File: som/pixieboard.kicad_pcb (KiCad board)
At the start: 8 copper layers, 50 x 50 mm, 11 parts, among them U1 XC7A200T-3FBG484E, U2 AS4C256M16D3, U3 AS4C256M16D3

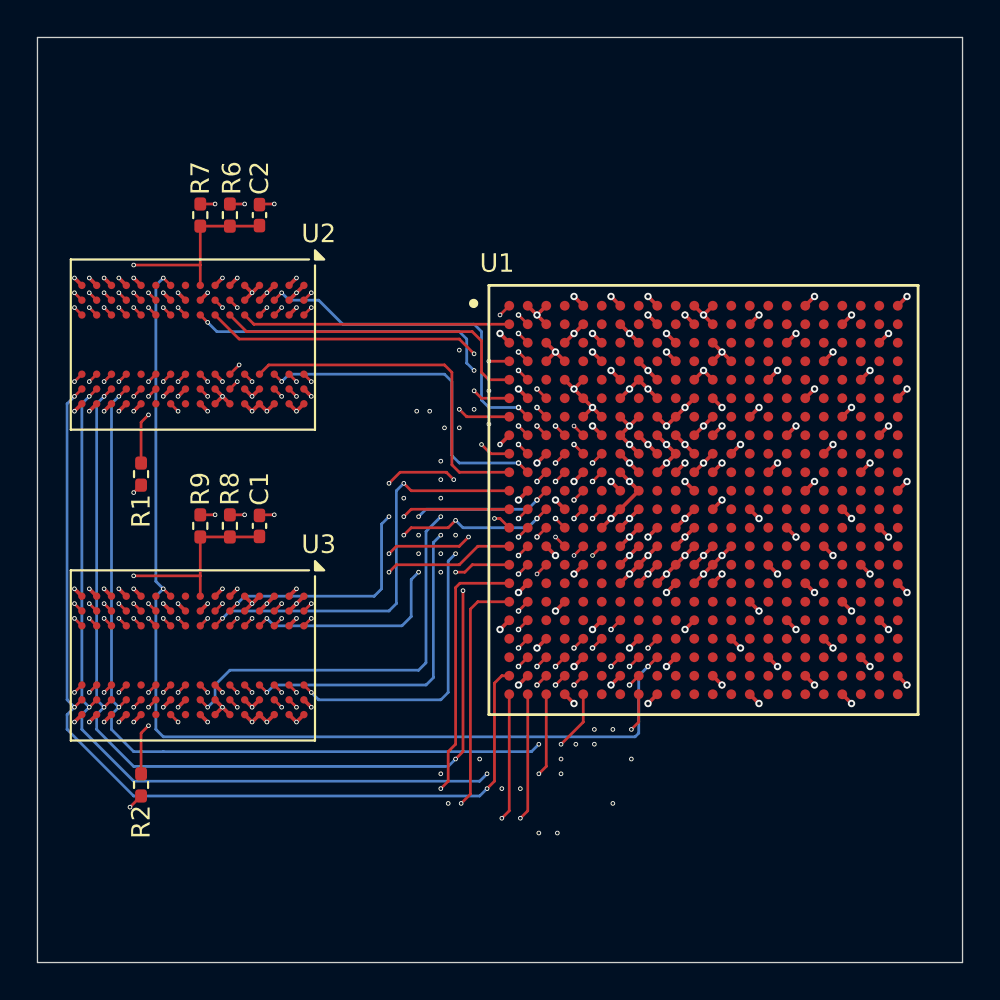
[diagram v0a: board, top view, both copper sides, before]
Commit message: lmfao l
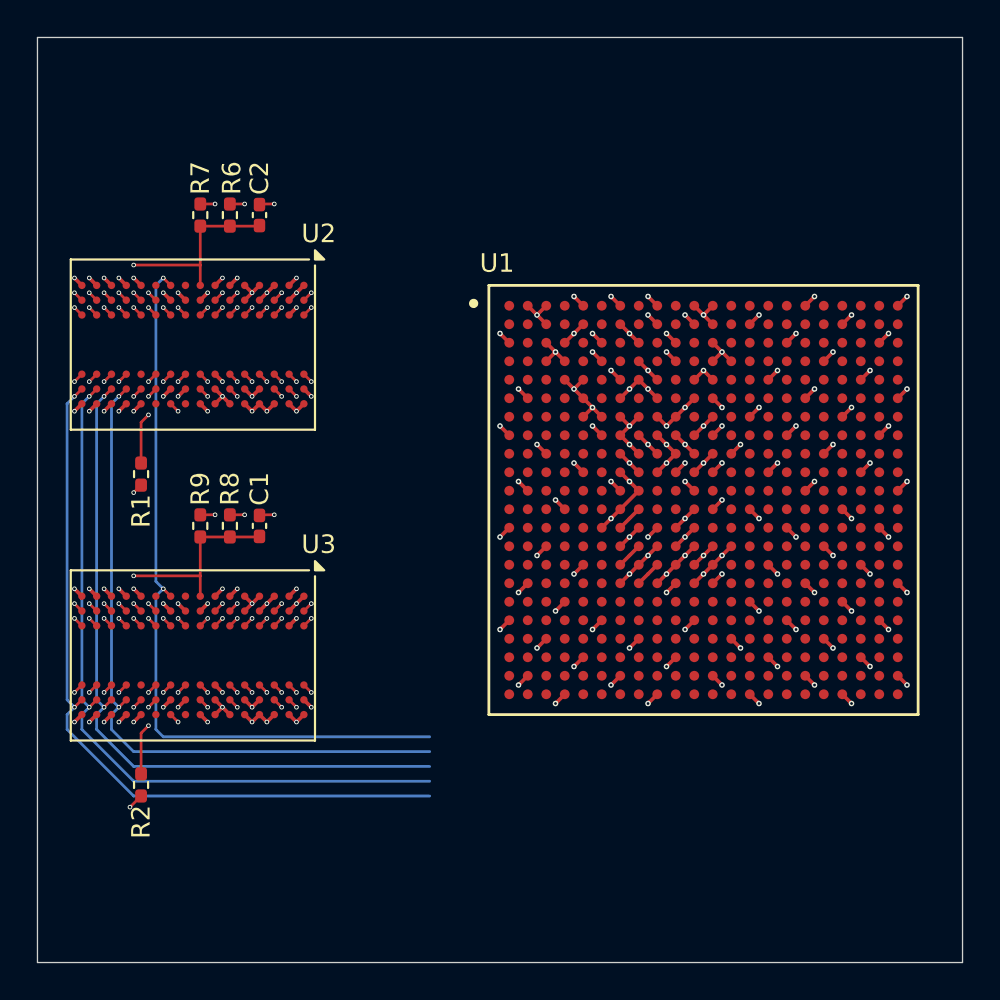
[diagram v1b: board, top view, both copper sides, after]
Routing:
- net /DDR3/DDR_D23: track 34.2 -> 0.57 mm, vias 3 -> 1
- net /DDR3/DDR_D17: track 28.9 -> 0.57 mm, vias 3 -> 1
- net /DDR3/DDR_D19: track 28.4 -> 0.57 mm, vias 2 -> 1
- net /DDR3/DDR_DM2: track 28.1 -> 0.57 mm, vias 3 -> 1
- net /DDR3/DDR_D22: track 27.9 -> 0.57 mm, vias 4 -> 1
- net /DDR3/DDR_D21: track 27.3 -> 0.57 mm, vias 3 -> 1
- net /DDR3/DDR_D30: track 26.2 -> 0.57 mm, vias 3 -> 1
- net /DDR3/DDR_D24: track 25.0 -> 0.57 mm, vias 3 -> 1
- net /DDR3/DDR_D16: track 23.8 -> 0.57 mm, vias 3 -> 1
- net /DDR3/DDR_D20: track 23.6 -> 0.57 mm, vias 4 -> 1
- net /DDR3/DDR_DQS3+: track 23.2 -> 0.57 mm, vias 3 -> 1
- net /DDR3/DDR_DQS2-: track 22.8 -> 0.57 mm, vias 2 -> 1
- net /DDR3/DDR_DQS3-: track 22.4 -> 0.57 mm, vias 3 -> 1
- net /DDR3/DDR_D18: track 22.2 -> 0.57 mm, vias 4 -> 1
- net /DDR3/DDR_DM3: track 21.8 -> 0.57 mm, vias 3 -> 1
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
